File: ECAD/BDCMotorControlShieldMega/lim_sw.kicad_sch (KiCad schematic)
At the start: 26 parts, among them J10 Limit switch, J11 Limit switch, J13 Limit switch, J14 Limit switch, J16 Limit switch, J17 Limit switch, U5 74AHC14

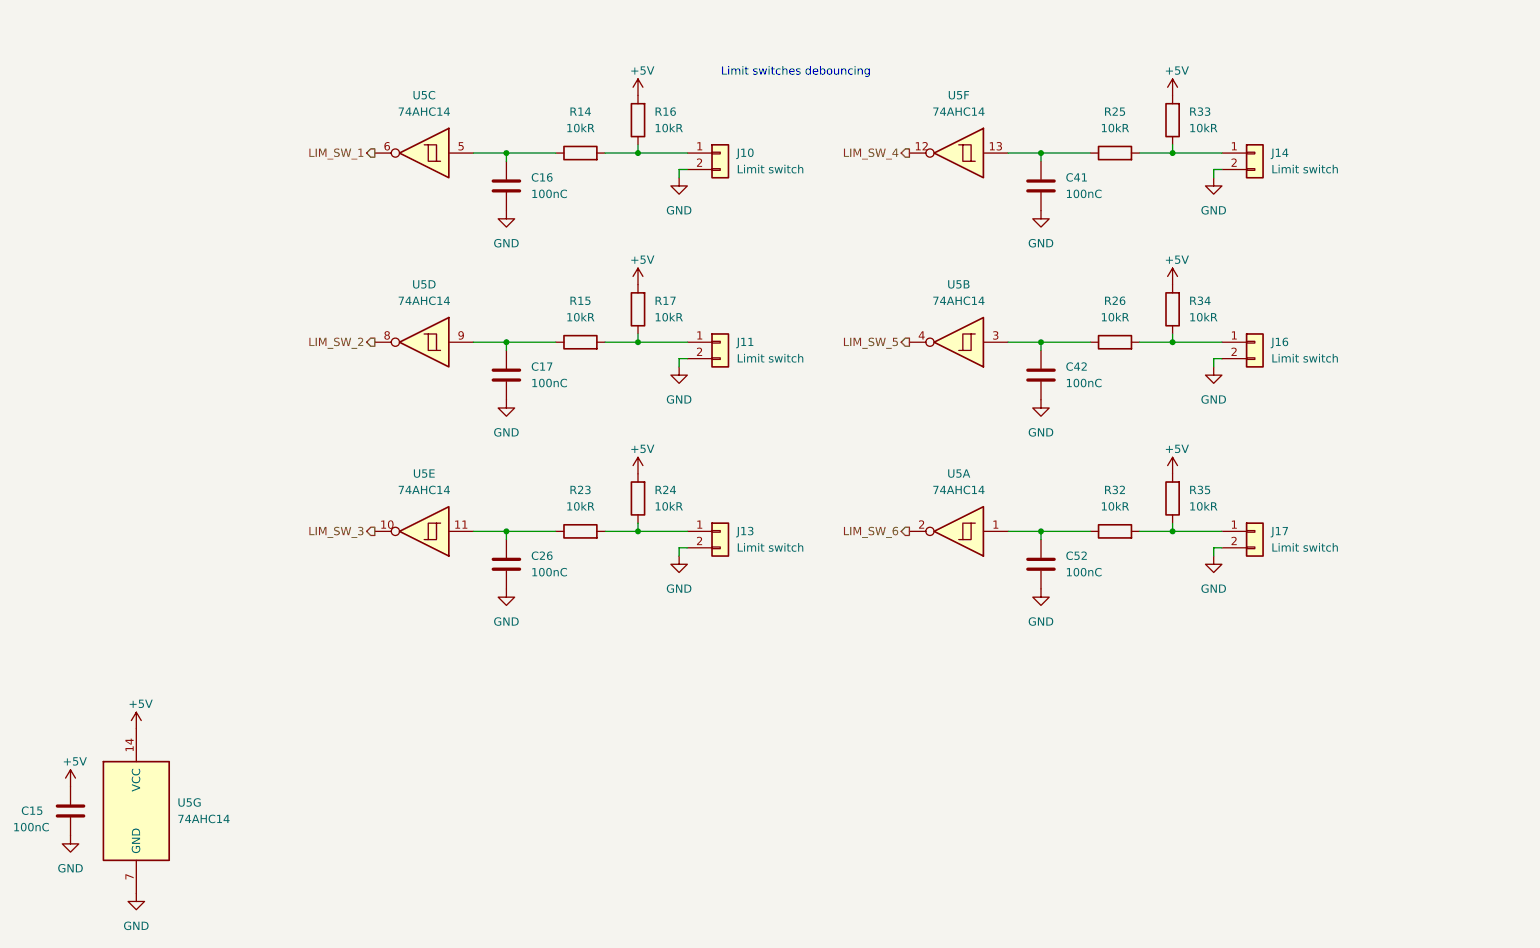
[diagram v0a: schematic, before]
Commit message: Progressed ECAD.
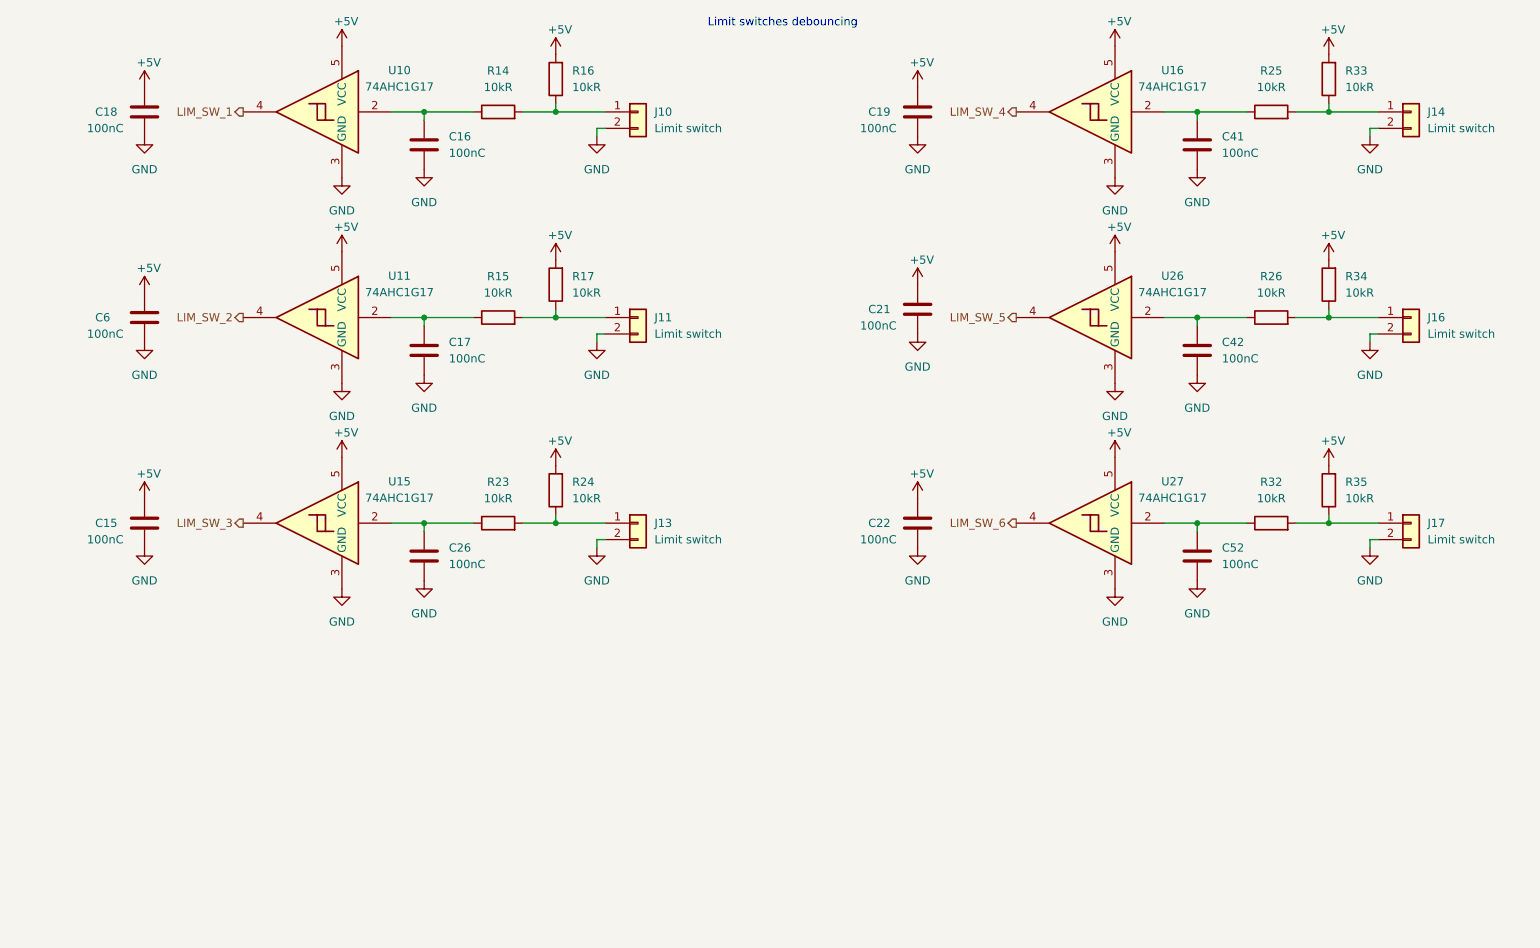
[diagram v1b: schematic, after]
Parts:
- removed U5: 74AHC14, Package_SO:TSSOP-14_4.4x5mm_P0.65mm, symbol 74xx:74HC14
- added C18, C19, C21, C22, C6: 100nC, Capacitor_SMD:C_0805_2012Metric, symbol Device:C
- added U10, U11, U15, U16, U26, U27: 74AHC1G17, Package_TO_SOT_SMD:SC-74A-5_1.55x2.9mm_P0.95mm, symbol 74xGxx:74LVC1G17
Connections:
- net +5V: now also C18.1, C19.1, C21.1, C22.1, C6.1, U10.5 (VCC), U11.5 (VCC), U15.5 (VCC), U16.5 (VCC), U26.5 (VCC), U27.5 (VCC)
- net GND: now also C18.2, C19.2, C21.2, C22.2, C6.2, U10.3 (GND), U11.3 (GND), U15.3 (GND), U16.3 (GND), U26.3 (GND), U27.3 (GND)
- net LIM_SW_1: now also U10.4
- net LIM_SW_2: now also U11.4
- net LIM_SW_3: now also U15.4
- net LIM_SW_4: now also U16.4
- net LIM_SW_5: now also U26.4
- net LIM_SW_6: now also U27.4
- net at C41.1, R25.1: now also U16.2
- net at C17.1, R15.1: now also U11.2
- net at C26.1, R23.1: now also U15.2
- net at C52.1, R32.1: now also U27.2
- net at C16.1, R14.1: now also U10.2
- net at C42.1, R26.1: now also U26.2
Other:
- moved on the sheet: C15, C16, C17, C26, C41, C42, C52, J10, J11, J13, J14, J16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

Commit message: Progressed ECAD.
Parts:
- C15, C16, C17, C18, C19, C21, C22, C26, C41, C42, C52, C6: footprint Capacitor_SMD:C_0805_2012Metric -> Capacitor_SMD:C_0603_1608Metric; MPN C0805F104K5RACAUTO -> (none)
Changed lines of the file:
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@@
 			)
 		)
-		(property "Footprint" "Capacitor_SMD:C_0805_2012Metric"
+		(property "Footprint" "Capacitor_SMD:C_0603_1608Metric"
 			(at 47.9552 63.5 0)
 			(effects
@@
 			)
 		)
-		(property "Datasheet" "https://www.lcsc.com/datasheet/lcsc_datasheet_2304140030_KEMET-C0805F104K5RACAUTO_C141162.pdf"
+		(property "Datasheet" ""
 			(at 46.99 59.69 0)
 			(effects
@@
 			)
 		)
-		(property "MPN" "C0805F104K5RACAUTO"
+		(property "MPN" ""
 			(at 46.99 59.69 0)
 			(effects
@@
 			)
 		)
-		(property "Footprint" "Capacitor_SMD:C_0805_2012Metric"
+		(property "Footprint" "Capacitor_SMD:C_0603_1608Metric"
 			(at 167.3352 127 0)
 			(effects
@@
 			)
 		)
-		(property "Datasheet" "https://www.lcsc.com/datasheet/lcsc_datasheet_2304140030_KEMET-C0805F104K5RACAUTO_C141162.pdf"
+		(property "Datasheet" ""
 			(at 166.37 123.19 0)
 			(effects
@@
 			)
 		)
-		(property "MPN" "C0805F104K5RACAUTO"
+		(property "MPN" ""
 			(at 166.37 123.19 0)
 			(effects
@@
 			)
 		)
-		(property "Footprint" "Capacitor_SMD:C_0805_2012Metric"
+		(property "Footprint" "Capacitor_SMD:C_0603_1608Metric"
 			(at 167.3352 63.5 0)
 			(effects
@@
 			)
 		)
-		(property "Datasheet" "https://www.lcsc.com/datasheet/lcsc_datasheet_2304140030_KEMET-C0805F104K5RACAUTO_C141162.pdf"
+		(property "Datasheet" ""
 			(at 166.37 59.69 0)
 			(effects
@@
 			)
 		)
-		(property "MPN" "C0805F104K5RACAUTO"
+		(property "MPN" ""
 			(at 166.37 59.69 0)
 			(effects
@@
 			)
 		)
-		(property "Footprint" "Capacitor_SMD:C_0805_2012Metric"
+		(property "Footprint" "Capacitor_SMD:C_0603_1608Metric"
 			(at 167.3352 93.98 0)
 			(effects
@@
 			)
 		)
-		(property "Datasheet" "https://www.lcsc.com/datasheet/lcsc_datasheet_2304140030_KEMET-C0805F104K5RACAUTO_C141162.pdf"
+		(property "Datasheet" ""
 			(at 166.37 90.17 0)
 			(effects
@@
 			)
 		)
-		(property "MPN" "C0805F104K5RACAUTO"
+		(property "MPN" ""
 			(at 166.37 90.17 0)
 			(effects
@@
 			)
 		)
-		(property "Footprint" "Capacitor_SMD:C_0805_2012Metric"
+		(property "Footprint" "Capacitor_SMD:C_0603_1608Metric"
 			(at 47.9552 127 0)
 			(effects
@@
 			)
 		)
-		(property "Datasheet" "https://www.lcsc.com/datasheet/lcsc_datasheet_2304140030_KEMET-C0805F104K5RACAUTO_C141162.pdf"
+		(property "Datasheet" ""
 			(at 46.99 123.19 0)
 			(effects
@@
 			)
 		)
-		(property "MPN" "C0805F104K5RACAUTO"
+		(property "MPN" ""
 			(at 46.99 123.19 0)
 			(effects
@@
 			)
 		)
-		(property "Footprint" "Capacitor_SMD:C_0805_2012Metric"
+		(property "Footprint" "Capacitor_SMD:C_0603_1608Metric"
 			(at 91.1352 132.08 0)
 			(effects
@@
 			)
 		)
-		(property "Datasheet" "https://www.lcsc.com/datasheet/lcsc_datasheet_2304140030_KEMET-C0805F104K5RACAUTO_C141162.pdf"
+		(property "Datasheet" ""
 			(at 90.17 128.27 0)
 			(effects
@@
 			)
 		)
-		(property "MPN" "C0805F104K5RACAUTO"
+		(property "MPN" ""
 			(at 90.17 128.27 0)
 			(effects
@@
 			)
 		)
-		(property "Footprint" "Capacitor_SMD:C_0805_2012Metric"
+		(property "Footprint" "Capacitor_SMD:C_0603_1608Metric"
 			(at 91.1352 100.33 0)
 			(effects
@@
 			)
 		)
-		(property "Datasheet" "https://www.lcsc.com/datasheet/lcsc_datasheet_2304140030_KEMET-C0805F104K5RACAUTO_C141162.pdf"
+		(property "Datasheet" ""
 			(at 90.17 96.52 0)
 			(effects
@@
 			)
 		)
-		(property "MPN" "C0805F104K5RACAUTO"
+		(property "MPN" ""
 			(at 90.17 96.52 0)
 			(effects
@@
 			)
 		)
-		(property "Footprint" "Capacitor_SMD:C_0805_2012Metric"
+		(property "Footprint" "Capacitor_SMD:C_0603_1608Metric"
 			(at 91.1352 68.58 0)
 			(effects
@@
 			)
 		)
-		(property "Datasheet" "https://www.lcsc.com/datasheet/lcsc_datasheet_2304140030_KEMET-C0805F104K5RACAUTO_C141162.pdf"
+		(property "Datasheet" ""
 			(at 90.17 64.77 0)
 			(effects
@@
 			)
 		)
-		(property "MPN" "C0805F104K5RACAUTO"
+		(property "MPN" ""
 			(at 90.17 64.77 0)
 			(effects
@@
 			)
 		)
-		(property "Footprint" "Capacitor_SMD:C_0805_2012Metric"
+		(property "Footprint" "Capacitor_SMD:C_0603_1608Metric"
 			(at 210.5152 100.33 0)
 			(effects
@@
 			)
 		)
-		(property "Datasheet" "https://www.lcsc.com/datasheet/lcsc_datasheet_2304140030_KEMET-C0805F104K5RACAUTO_C141162.pdf"
+		(property "Datasheet" ""
 			(at 209.55 96.52 0)
 			(effects
@@
 			)
 		)
-		(property "MPN" "C0805F104K5RACAUTO"
+		(property "MPN" ""
 			(at 209.55 96.52 0)
 			(effects
@@
 			)
 		)
-		(property "Footprint" "Capacitor_SMD:C_0805_2012Metric"
+		(property "Footprint" "Capacitor_SMD:C_0603_1608Metric"
 			(at 210.5152 132.08 0)
 			(effects
@@
 			)
 		)
-		(property "Datasheet" "https://www.lcsc.com/datasheet/lcsc_datasheet_2304140030_KEMET-C0805F104K5RACAUTO_C141162.pdf"
+		(property "Datasheet" ""
 			(at 209.55 128.27 0)
 			(effects
@@
 			)
 		)
-		(property "MPN" "C0805F104K5RACAUTO"
+		(property "MPN" ""
 			(at 209.55 128.27 0)
 			(effects
@@
 			)
 		)
-		(property "Footprint" "Capacitor_SMD:C_0805_2012Metric"
+		(property "Footprint" "Capacitor_SMD:C_0603_1608Metric"
 			(at 210.5152 68.58 0)
 			(effects
@@
 			)
 		)
-		(property "Datasheet" "https://www.lcsc.com/datasheet/lcsc_datasheet_2304140030_KEMET-C0805F104K5RACAUTO_C141162.pdf"
+		(property "Datasheet" ""
 			(at 209.55 64.77 0)
 			(effects
@@
 			)
 		)
-		(property "MPN" "C0805F104K5RACAUTO"
+		(property "MPN" ""
 			(at 209.55 64.77 0)
 			(effects
@@
 			)
 		)
-		(property "Footprint" "Capacitor_SMD:C_0805_2012Metric"
+		(property "Footprint" "Capacitor_SMD:C_0603_1608Metric"
 			(at 47.9552 95.25 0)
 			(effects
@@
 			)
 		)
-		(property "Datasheet" "https://www.lcsc.com/datasheet/lcsc_datasheet_2304140030_KEMET-C0805F104K5RACAUTO_C141162.pdf"
+		(property "Datasheet" ""
 			(at 46.99 91.44 0)
 			(effects
@@
 			)
 		)
-		(property "MPN" "C0805F104K5RACAUTO"
+		(property "MPN" ""
 			(at 46.99 91.44 0)
 			(effects

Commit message: Progressed ECAD.
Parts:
- C15, C16, C17, C18, C19, C21, C22, C26, C41, C42, C52, C6: footprint Capacitor_SMD:C_0603_1608Metric -> Capacitor_SMD:C_0805_2012Metric
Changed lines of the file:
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@@
 			)
 		)
-		(property "Footprint" "Capacitor_SMD:C_0603_1608Metric"
+		(property "Footprint" "Capacitor_SMD:C_0805_2012Metric"
 			(at 47.9552 63.5 0)
 			(effects
@@
 			)
 		)
-		(property "Footprint" "Capacitor_SMD:C_0603_1608Metric"
+		(property "Footprint" "Capacitor_SMD:C_0805_2012Metric"
 			(at 167.3352 127 0)
 			(effects
@@
 			)
 		)
-		(property "Footprint" "Capacitor_SMD:C_0603_1608Metric"
+		(property "Footprint" "Capacitor_SMD:C_0805_2012Metric"
 			(at 167.3352 63.5 0)
 			(effects
@@
 			)
 		)
-		(property "Footprint" "Capacitor_SMD:C_0603_1608Metric"
+		(property "Footprint" "Capacitor_SMD:C_0805_2012Metric"
 			(at 167.3352 93.98 0)
 			(effects
@@
 			)
 		)
-		(property "Footprint" "Capacitor_SMD:C_0603_1608Metric"
+		(property "Footprint" "Capacitor_SMD:C_0805_2012Metric"
 			(at 47.9552 127 0)
 			(effects
@@
 			)
 		)
-		(property "Footprint" "Capacitor_SMD:C_0603_1608Metric"
+		(property "Footprint" "Capacitor_SMD:C_0805_2012Metric"
 			(at 91.1352 132.08 0)
 			(effects
@@
 			)
 		)
-		(property "Footprint" "Capacitor_SMD:C_0603_1608Metric"
+		(property "Footprint" "Capacitor_SMD:C_0805_2012Metric"
 			(at 91.1352 100.33 0)
 			(effects
@@
 			)
 		)
-		(property "Footprint" "Capacitor_SMD:C_0603_1608Metric"
+		(property "Footprint" "Capacitor_SMD:C_0805_2012Metric"
 			(at 91.1352 68.58 0)
 			(effects
@@
 			)
 		)
-		(property "Footprint" "Capacitor_SMD:C_0603_1608Metric"
+		(property "Footprint" "Capacitor_SMD:C_0805_2012Metric"
 			(at 210.5152 100.33 0)
 			(effects
@@
 			)
 		)
-		(property "Footprint" "Capacitor_SMD:C_0603_1608Metric"
+		(property "Footprint" "Capacitor_SMD:C_0805_2012Metric"
 			(at 210.5152 132.08 0)
 			(effects
@@
 			)
 		)
-		(property "Footprint" "Capacitor_SMD:C_0603_1608Metric"
+		(property "Footprint" "Capacitor_SMD:C_0805_2012Metric"
 			(at 210.5152 68.58 0)
 			(effects
@@
 			)
 		)
-		(property "Footprint" "Capacitor_SMD:C_0603_1608Metric"
+		(property "Footprint" "Capacitor_SMD:C_0805_2012Metric"
 			(at 47.9552 95.25 0)
 			(effects
